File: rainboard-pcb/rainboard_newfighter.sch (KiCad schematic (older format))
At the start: 98 parts, among them J1 Conn_01x02, J10 Conn_01x03, J11 SDS-50J, J12 SDS-50J, J13 Conn_01x02, J14 Conn_01x02, J15 Conn_01x02, J16 Conn_01x02, J17 Conn_01x02, J18 Conn_01x02, J2 Conn_01x02, J3 Conn_01x02, J4 Conn_01x02, J5 Conn_01x02, J6 Conn_01x02, J7 Conn_01x02, J8 Conn_01x02, J9 Conn_01x03, U1 MCP23017-E_SO, U2 74HC14D, U3 EL357N(A)(TA)-G

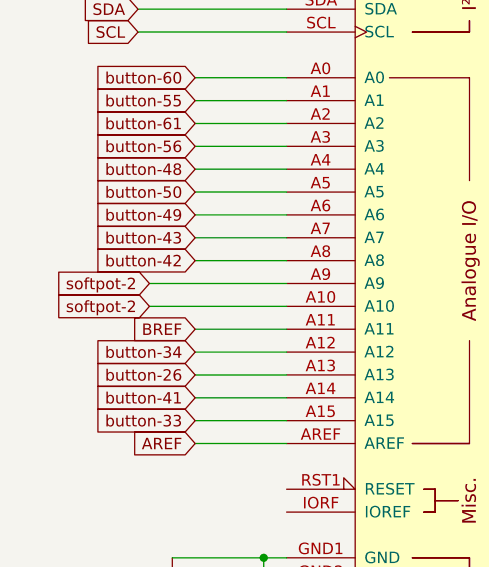
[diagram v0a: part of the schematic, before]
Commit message: start on v0.4 of PCB
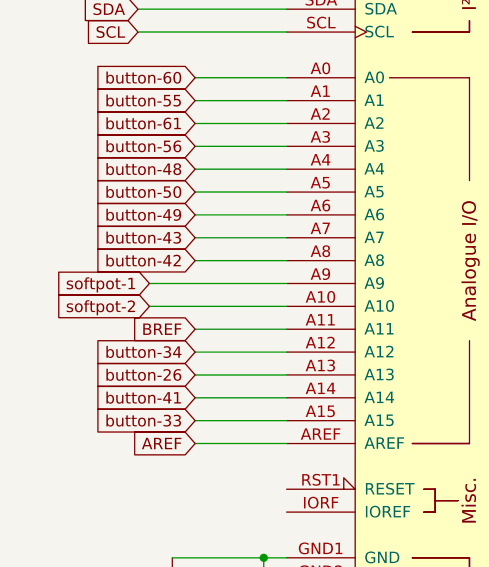
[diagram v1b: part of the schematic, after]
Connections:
- net softpot-1: now also XA1.A9
- net softpot-2: no longer XA1.A9
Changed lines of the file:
@@
 5V
 Text GLabel 1050 3250 0    50   Input ~ 0
-softpot-2
+softpot-1
 Wire Wire Line
 	1050 3250 1650 3250
